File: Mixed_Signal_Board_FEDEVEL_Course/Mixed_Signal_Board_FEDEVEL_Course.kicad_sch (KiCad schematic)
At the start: 0 parts

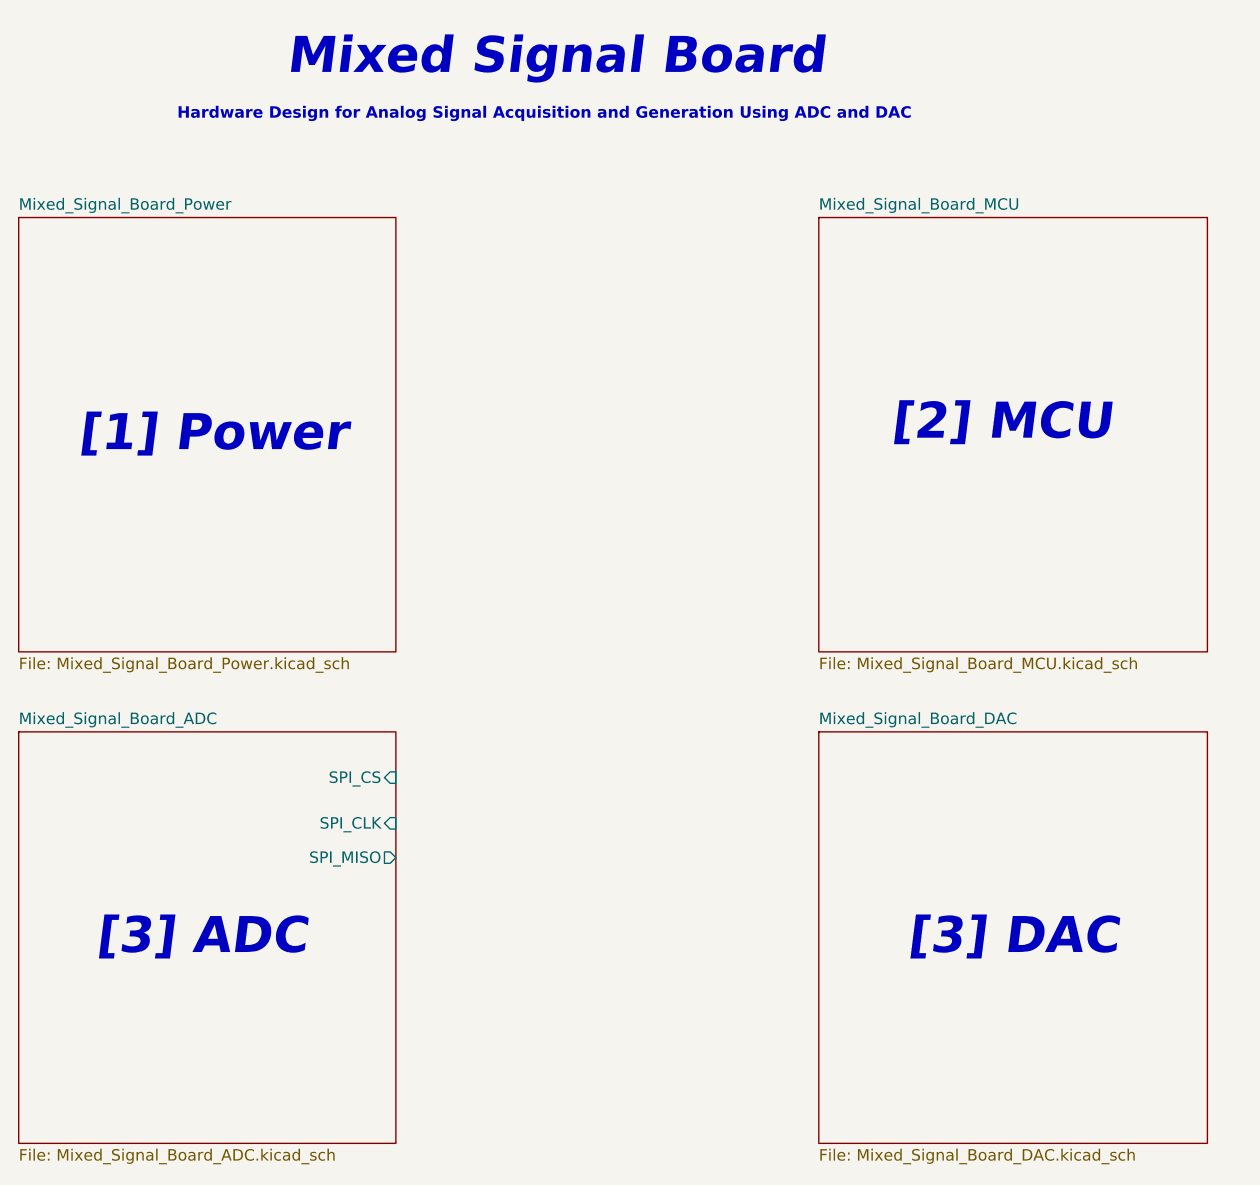
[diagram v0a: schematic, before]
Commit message: Handle the connections between sheets
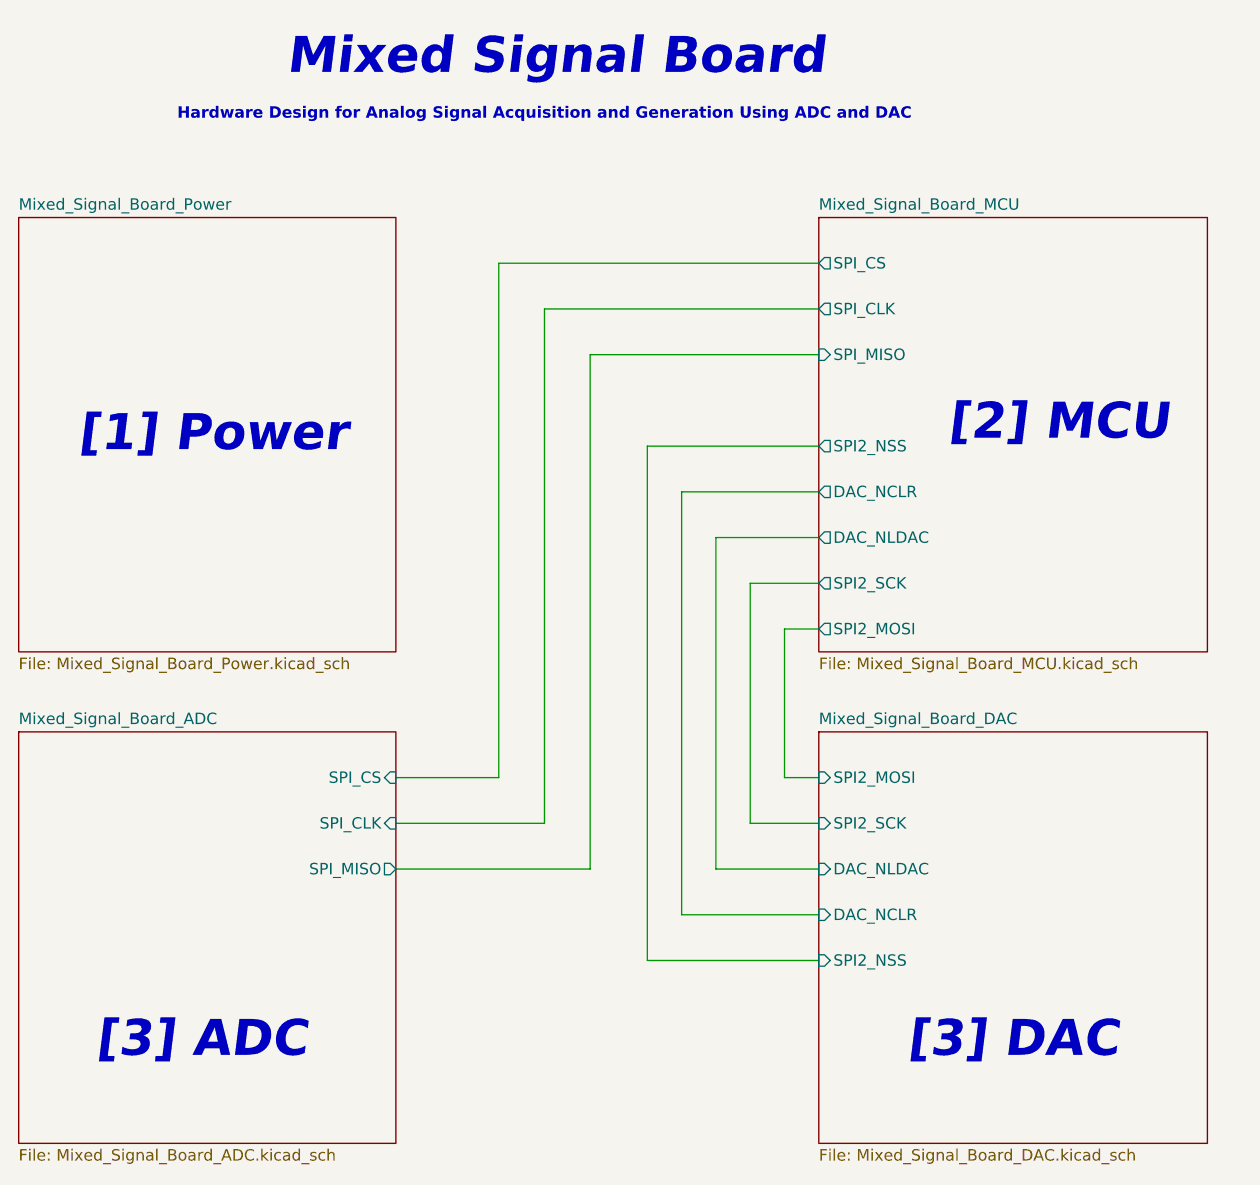
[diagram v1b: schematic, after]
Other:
- sheet Mixed_Signal_Board_DAC ports: added DAC_NCLR, DAC_NLDAC, SPI2_MOSI, SPI2_NSS, SPI2_SCK; removed none
- sheet Mixed_Signal_Board_MCU ports: added DAC_NCLR, DAC_NLDAC, SPI2_MOSI, SPI2_NSS, SPI2_SCK, SPI_CLK, SPI_CS, SPI_MISO; removed none
